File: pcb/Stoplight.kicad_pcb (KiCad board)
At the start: 2 copper layers, 15 x 15 mm, 18 parts, among them IC1 ATtiny85-20M, IC2 AP7375-33SA-7

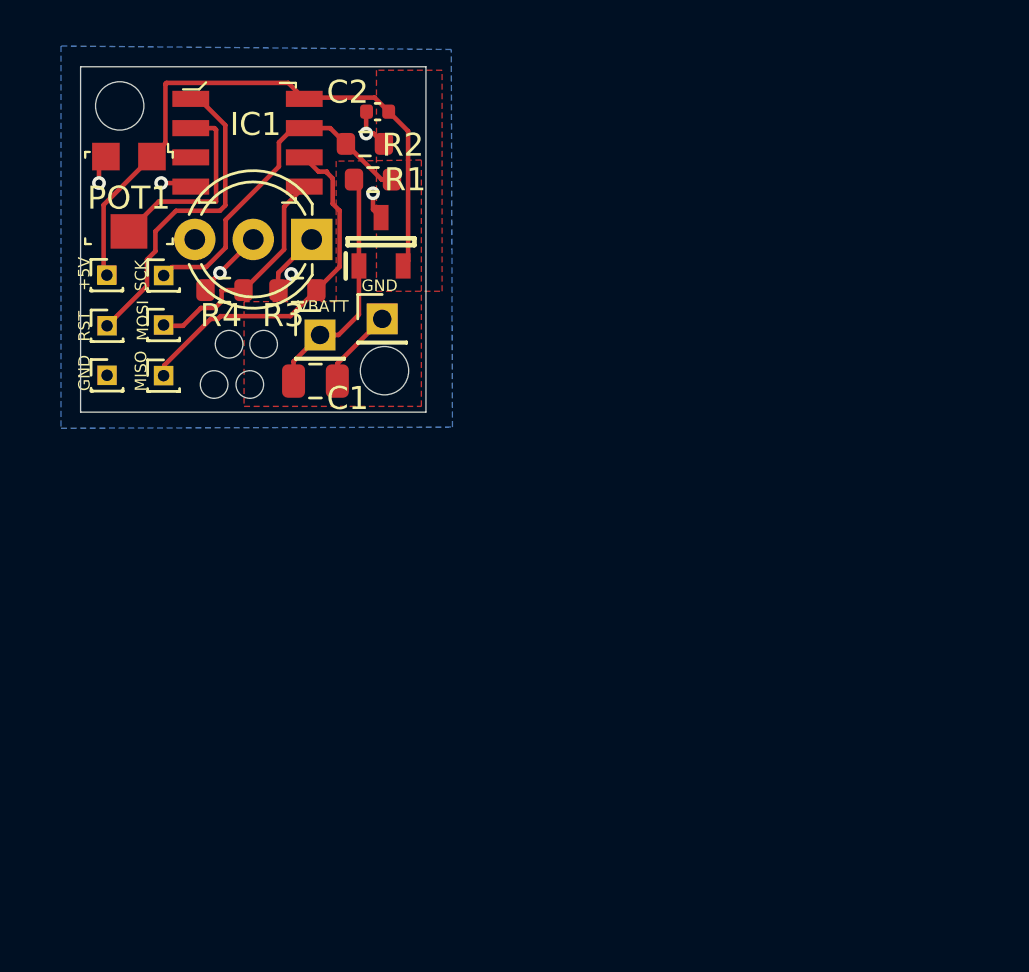
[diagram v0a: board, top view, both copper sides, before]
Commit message: pcb v1a
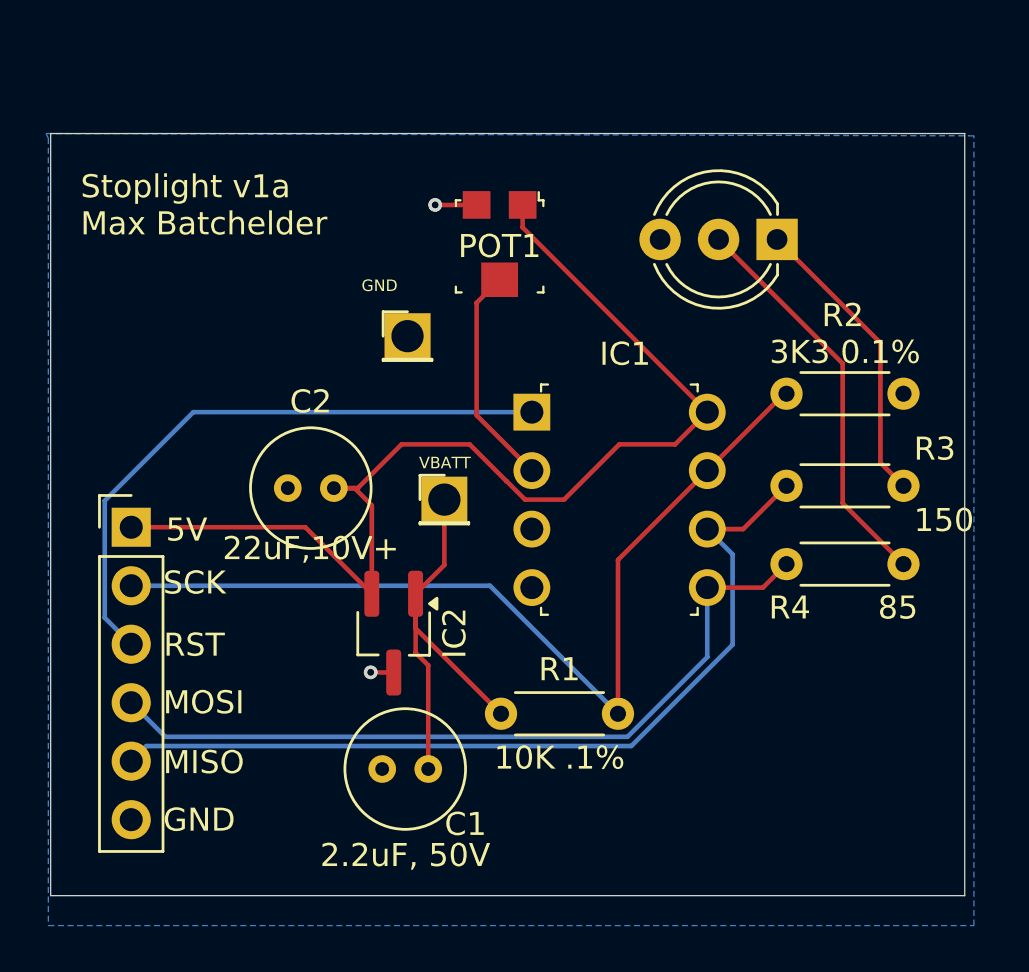
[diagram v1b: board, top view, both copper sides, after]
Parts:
- removed TP3: GND, Connector_PinHeader_1.00mm:PinHeader_1x01_P1.00mm_Vertical
- removed TP4: 3V3, Connector_PinHeader_1.00mm:PinHeader_1x01_P1.00mm_Vertical
- removed TP5: MISO, Connector_PinHeader_1.00mm:PinHeader_1x01_P1.00mm_Vertical
- removed TP6: MOSI, Connector_PinHeader_1.00mm:PinHeader_1x01_P1.00mm_Vertical
- removed TP7: SCK, Connector_PinHeader_1.00mm:PinHeader_1x01_P1.00mm_Vertical
- removed TP8: RST, Connector_PinHeader_1.00mm:PinHeader_1x01_P1.00mm_Vertical
- added REF**: PinHeader_1x06_P2.54mm_Vertical, Connector_PinHeader_2.54mm:PinHeader_1x06_P2.54mm_Vertical, F.Cu at (127.4, 99.6)
- C1: footprint Capacitor_SMD:C_0805_2012Metric -> Capacitor_THT:C_Radial_D5.0mm_H5.0mm_P2.00mm
- C2: footprint Capacitor_SMD:C_0402_1005Metric -> Capacitor_THT:C_Radial_D5.0mm_H5.0mm_P2.00mm
- IC1: footprint digikey-footprints:SOIC-8_W5.3mm -> digikey-footprints:DIP-8_W7.62mm
- IC2: footprint AP7375-33SA-7:SOT96P240X110-3N -> Package_TO_SOT_SMD:TSOT-23_HandSoldering
- R1, R2, R3, R4: footprint Resistor_SMD:R_0603_1608Metric -> Resistor_THT:R_Axial_DIN0204_L3.6mm_D1.6mm_P5.08mm_Horizontal
- moved R4 31.8 mm to (160.9, 101.2), turned to 180 degrees
- moved R3 27.7 mm to (160.9, 97.8), turned to 180 degrees
- moved R1 23.9 mm to (143.5, 107.7)
- moved R2 21.3 mm to (155.9, 93.8)
- moved D1 20.2 mm to (155.4, 87.1)
- moved C1 17.1 mm to (138.3, 110.1), turned to 0 degrees
- moved IC1 17.0 mm to (144.8, 94.6)
- moved IC2 17.0 mm to (138.8, 104.2), turned to -90 degrees
- moved C2 16.8 mm to (134.2, 97.9)
- moved POT1 16.2 mm to (143.4, 87.4)
- moved TP1 8.96 mm to (141.0, 98.4)
- moved TP2 1.33 mm to (139.4, 91.3)
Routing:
- net SCK/BATT: track 14.8 -> 40.4 mm
- net MOSI/R: track 10.0 -> 33.9 mm
- net +5V: track 26.9 -> 49.3 mm
- net MISO/G: track 15.5 -> 37.9 mm
- net Net-(D1-A2): track 3.06 -> 17.4 mm, vias 1 -> 0
- net RST: track 13.9 -> 26.9 mm
- net Net-(D1-A1): track 3.77 -> 13.0 mm, vias 1 -> 0
- net +VBATT: track 10.5 -> 19.2 mm
- net GND: track 9.24 -> 2.80 mm, vias 4 -> 2
- net DIM: track 8.57 -> 9.70 mm
- removed copper zone on F.Cu, net +5V
- removed copper zone on F.Cu, net +VBATT
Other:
- board size 15 x 15 mm -> 39.7 x 33.1 mm
- board text added: "5V"
- board text added: "Stoplight v1a Max Batchelder"
- board text removed: "+5V"
- board text removed: "Stoplight v1 Max Batchelder"
